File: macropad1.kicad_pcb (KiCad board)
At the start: 2 copper layers, 119.9 x 63.5 mm, 43 parts, among them J1 Conn_01x04, SW1 SW_Reed, SW2 Rotary_Encoder_Switch, U1 ATmega32U4-AU, Y1 16Mhz

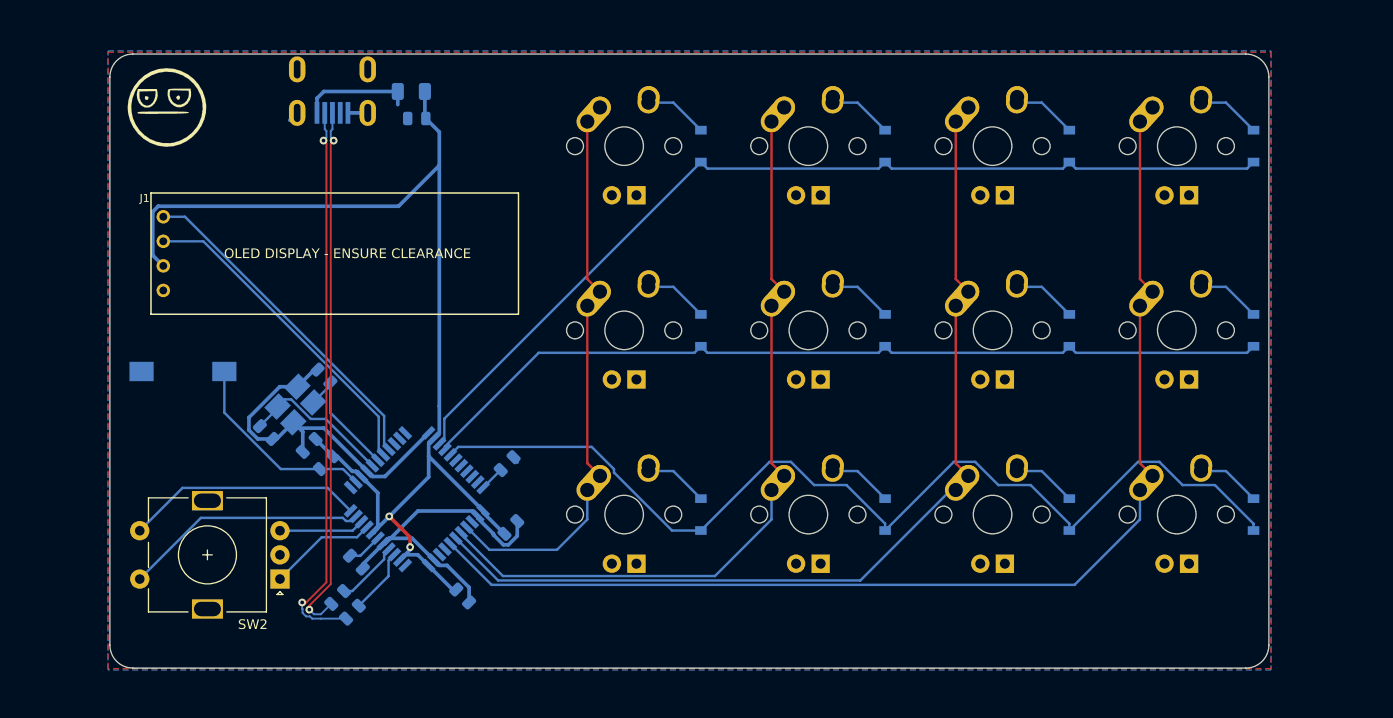
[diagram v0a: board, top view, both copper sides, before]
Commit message: Ready for prototyping
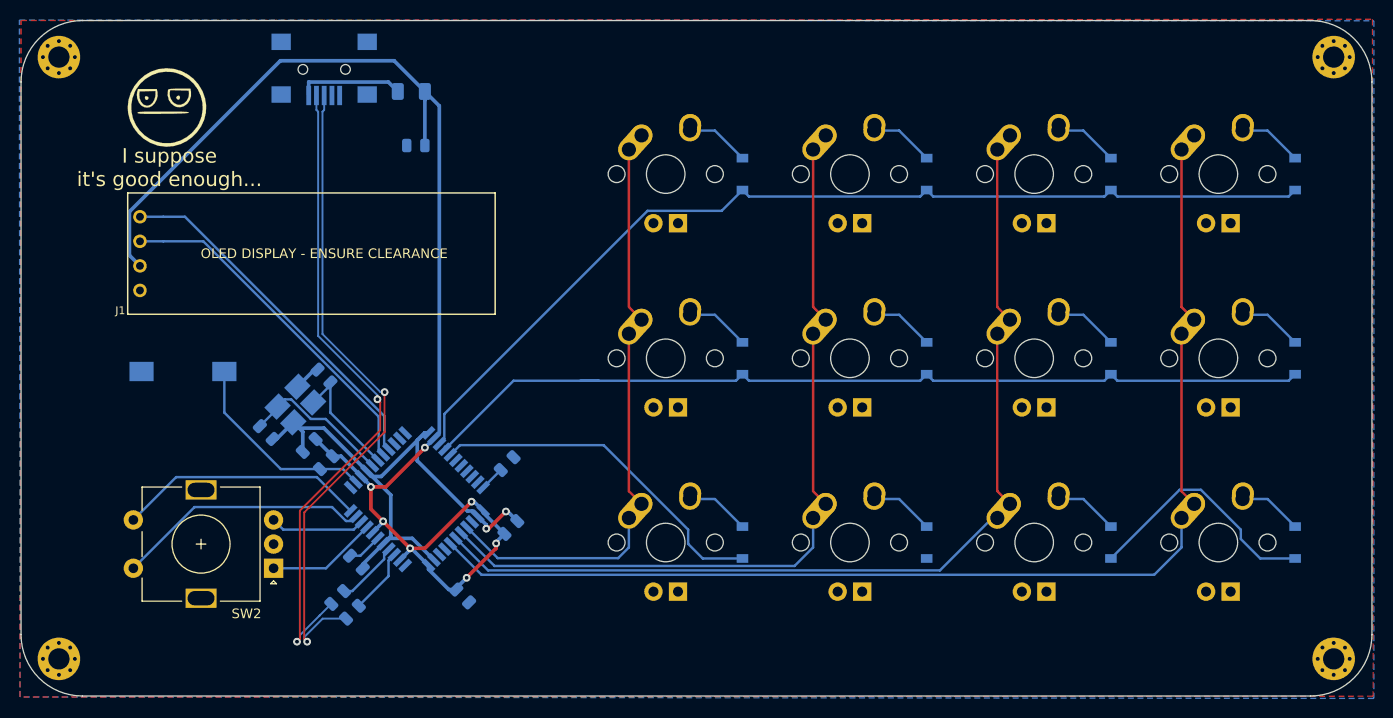
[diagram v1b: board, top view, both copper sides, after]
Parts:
- removed USB1: Molex-0548190589, random-keyboard-parts:Molex-0548190589
- added GND: MountingHole_2.2mm_M2_Pad_Via, MountingHole:MountingHole_2.2mm_M2_Pad_Via, F.Cu at (37.6, 24.1)
- added GND: MountingHole_2.2mm_M2_Pad_Via, MountingHole:MountingHole_2.2mm_M2_Pad_Via, F.Cu at (37.6, 86.4)
- added GND: MountingHole_2.2mm_M2_Pad_Via, MountingHole:MountingHole_2.2mm_M2_Pad_Via, F.Cu at (169.4, 86.4)
- added GND: MountingHole_2.2mm_M2_Pad_Via, MountingHole:MountingHole_2.2mm_M2_Pad_Via, F.Cu at (169.4, 24.1)
- added J2: USB_B_Mini, Connector_USB:USB_Mini-B_Lumberg_2486_01_Horizontal, B.Cu at (65.0, 25.4)
- moved D12 5.18 mm to (165.4, 74.3)
- moved D4 5.18 mm to (165.4, 36.2)
- moved D8 5.18 mm to (165.4, 55.3)
- moved MX12 5.18 mm to (157.5, 74.3)
- moved MX4 5.18 mm to (157.5, 36.2)
- moved MX8 5.18 mm to (157.5, 55.3)
- moved D1 5.18 mm to (108.3, 36.2)
- moved D10 5.18 mm to (127.3, 74.3)
- moved D2 5.18 mm to (127.3, 36.2)
- moved D5 5.18 mm to (108.3, 55.3)
- moved D6 5.18 mm to (127.3, 55.3)
- moved D9 5.18 mm to (108.3, 74.3)
- moved MX1 5.18 mm to (100.3, 36.2)
- moved MX10 5.18 mm to (119.4, 74.3)
- moved MX2 5.18 mm to (119.4, 36.2)
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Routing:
- net /ROW_2: track 106.1 -> 61.8 mm
- net +5V: track 125.5 -> 142.3 mm, vias 2 -> 7
- net GND: track 77.9 -> 64.2 mm, vias 0 -> 2
- net D+: track 55.5 -> 68.2 mm
- net D-: track 58.1 -> 68.7 mm
- net /ROW_1: track 90.1 -> 95.2 mm
- net /COL_0: track 54.0 -> 57.9 mm
- net /ROW_0: track 99.2 -> 102.5 mm
- net /SDA: track 35.0 -> 37.4 mm
- net /SCL: track 33.9 -> 36.3 mm
- net /COL_3: track 115.2 -> 117.4 mm
- net /COL_2: track 93.6 -> 95.9 mm
- net /COL_1: track 75.8 -> 77.9 mm
- net /ENC_S2: track 25.3 -> 26.4 mm
- net /ENC_S1: track 24.6 -> 25.7 mm
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- added copper zone on F.Cu, net (none)
- removed copper zone on F.Cu, net GND
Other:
- board size 119.9 x 63.5 mm -> 139.7 x 69.8 mm
- board text added: "I suppose it's good enough..."
